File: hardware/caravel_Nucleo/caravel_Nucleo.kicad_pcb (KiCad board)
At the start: 2 copper layers, 67 x 92.4 mm, 80 parts, among them J1 USB_B_Micro - 10118193-0001LF, J10 Conn_01x09_Female, J2 Conn_01x02_Female, J3 Conn_01x02_Male, J4 Conn_01x04_Female, J5 Conn_01x02_Male, J6 Conn_01x02_Male, J7 Conn_01x06_Female, J8 Conn_01x03, J9 Conn_01x03, SW1 SW_Push - SKQGADE010, T1 Logo, T2 Logo, U1 FT232H, U10 MCP4661, U11 NUCLEO144-F429ZI, U2 SN74LVC1G125DCKR, U3 SN74LVC1G125DCKR, U4 MCP1319MT-29LE-OT, U5 TAR5SxxU_SOT353F, U6 TAR5SxxU_SOT353F, U7 W25Q32FVSS, U8 caravel_breakout, U9 MIC2211-AAYML-TR, X1 DSC6001_10MHZ, Y1 CSTNE12M0GH5L000R0

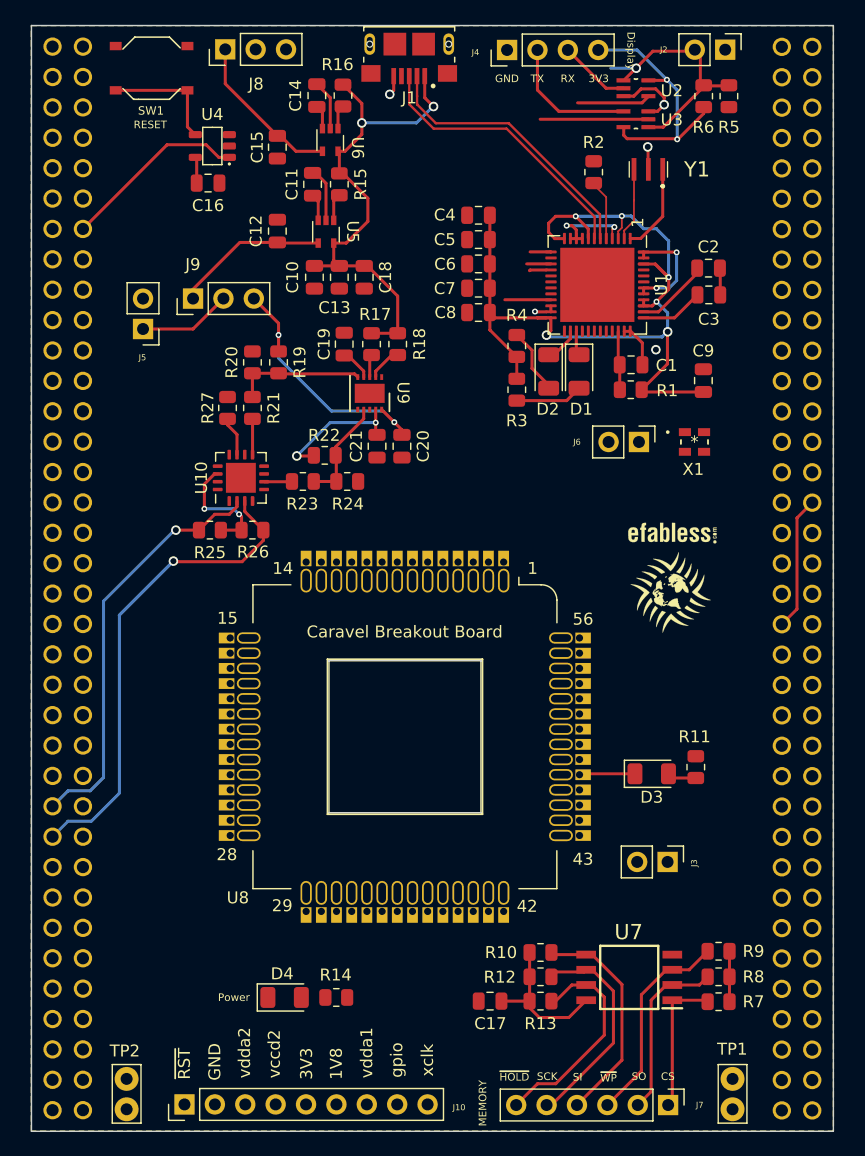
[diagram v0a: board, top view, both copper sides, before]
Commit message: [in review] update caravel board Nucleo-144 hat
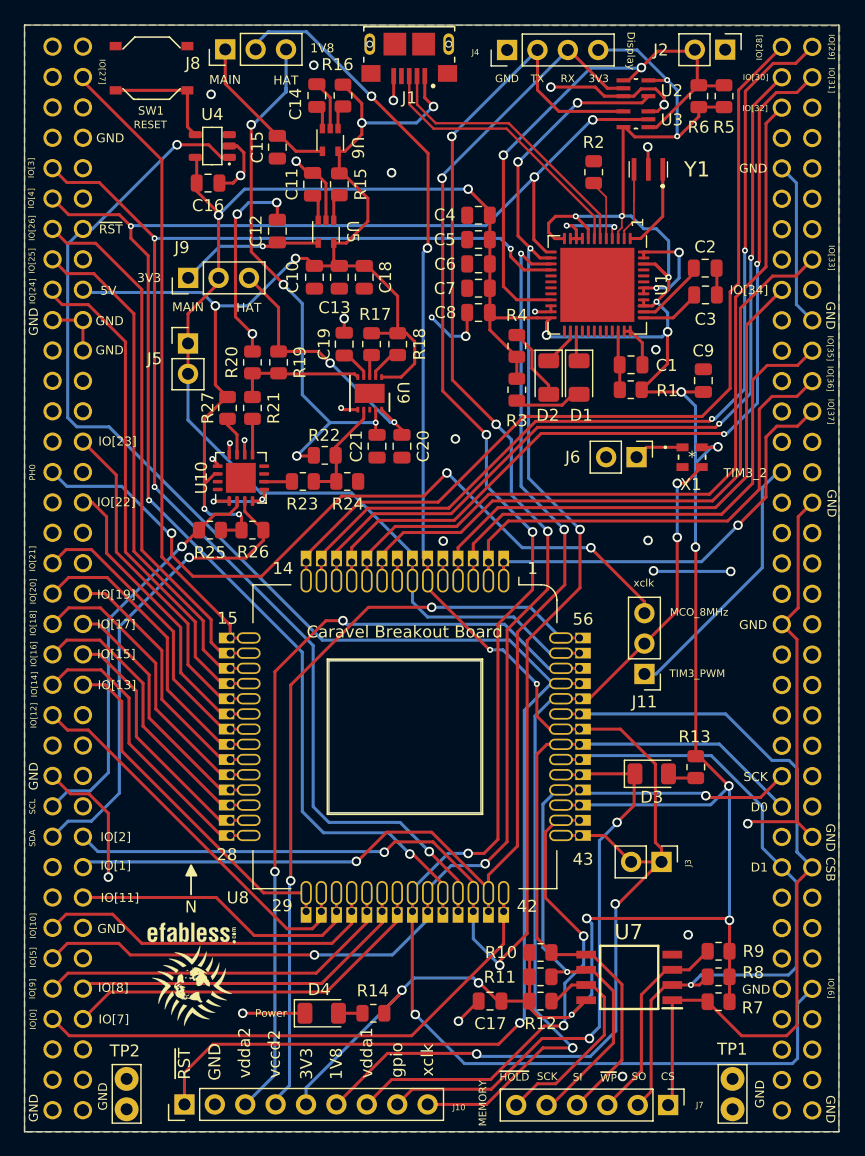
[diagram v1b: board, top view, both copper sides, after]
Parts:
- added J11: Conn_01x03, Connector_PinHeader_2.54mm:PinHeader_1x03_P2.54mm_Vertical, F.Cu at (146.9, 123.0)
- moved T2 52.3 mm to (109.0, 144.6)
- moved T1 51.8 mm to (109.0, 149.0)
- moved J5 3.95 mm to (108.7, 95.3), turned to 0 degrees
- moved D4 3.37 mm to (119.9, 151.3)
- moved R14 3.37 mm to (124.2, 151.3)
- moved J9 1.77 mm to (108.7, 89.9)
- moved X1 1.29 mm to (150.8, 104.9)
- moved J6 1.29 mm to (146.2, 104.9)
- moved J3 0.51 mm to (148.3, 138.7)
- moved D1 0.51 mm to (141.4, 98.2)
- moved D2 0.51 mm to (138.9, 98.2)
- moved R5 0.41 mm to (153.5, 74.7)
- moved R6 0.41 mm to (151.4, 74.7)
- moved C3 0.28 mm to (152.0, 91.3)
- moved C2 0.28 mm to (151.9, 89.1)
- renumbered R12 to R11, R13 to R12, R11 to R13
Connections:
- J10 pad 9: TIM3_CH2 -> xclk
- J3 pad 2: vccd1 -> vccd
- J4 pad 2: UART3_TX -> UART8_TX
- J4 pad 3: UART3_RX -> UART8_RX
- J5 pad 2: vddio -> vdda
- U1 pad 13: USB_SCK_TXD -> SPI5_SCK
- U1 pad 14: USB_SO_RXD -> SPI5_MISO
- U1 pad 15: USB_SI -> SPI5_MOSI
- U1 pad 16: USB_CS1 -> SPI5_CS
- U11 pad 1: UART3_TX -> unconnected-(U11-Pad1)
- U11 pad 136: unconnected-(U11-Pad136) -> UART8_RX
- U11 pad 2: UART3_RX -> unconnected-(U11-Pad2)
- U11 pad 29: unconnected-(U11-Pad29) -> PH0
- U11 pad 61: unconnected-(U11-Pad61) -> UART8_TX
- U2 pad 2: UART3_RX -> UART8_RX
- U2 pad 4: USB_SO_RXD -> SPI5_MISO
- U3 pad 2: USB_SCK_TXD -> SPI5_SCK
- U3 pad 4: UART3_TX -> UART8_TX
- U8 pad 36: UART3_RX -> UART8_RX
- U8 pad 37: UART3_TX -> UART8_TX
- U8 pad 38: USB_SCK_TXD -> SPI5_SCK
- U8 pad 39: USB_CS1 -> SPI5_CS
- U8 pad 40: USB_SO_RXD -> SPI5_MISO
- U8 pad 41: USB_SI -> SPI5_MOSI
- U8 pad 43: vccd1 -> vccd
- U8 pad 52: TIM3_CH2 -> xclk
- U8 pad 55: vddio -> vdda
- U8 pad 7: vddio -> vdda
- X1 pad 3: TIM3_CH2 -> xclk
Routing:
- net vdda: track 125.8 -> 328.0 mm, vias 8 -> 19
- net vccd: track 0.00 -> 142.7 mm, vias 0 -> 6
- net UART8_RX: track 0.00 -> 140.3 mm, vias 0 -> 5
- net SPI5_SCK: track 0.00 -> 132.6 mm, vias 0 -> 5
- net ~{RST}: track 15.6 -> 146.6 mm, vias 0 -> 2
- net SPI5_MISO: track 0.00 -> 130.2 mm, vias 0 -> 6
- net UART8_TX: track 0.00 -> 129.5 mm, vias 0 -> 5
- net GND: track 54.1 -> 174.2 mm, vias 9 -> 38
- net SPI5_CS: track 0.00 -> 114.8 mm, vias 0 -> 4
- net SPI5_MOSI: track 0.00 -> 99.4 mm, vias 0 -> 3
- net mprj_io[29]: track 0.00 -> 75.3 mm, vias 0 -> 2
- net mprj_io[28]: track 0.00 -> 73.7 mm
- net xclk: track 0.00 -> 71.9 mm, vias 0 -> 3
- net mprj_io[31]: track 0.00 -> 71.9 mm, vias 0 -> 2
- net mprj_io[30]: track 0.00 -> 70.1 mm, vias 0 -> 2
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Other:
- board size 67 x 92.4 mm -> 68.1 x 92.5 mm
- board text added: "5V"
- board text added: "CSB"
- board text added: "D0"
- board text added: "D1"
- board text added: "HAT"
- board text added: "IO[0]"
- board text added: "IO[10]"
- board text added: "IO[11]"
- board text added: "IO[12]"
- board text added: "IO[13]"
- board text added: "IO[14]"
- board text added: "IO[15]"
- board text added: "IO[16]"
- board text added: "IO[17]"
- board text added: "IO[18]"
- board text added: "IO[19]"
- board text added: "IO[1]"
- board text added: "IO[20]"
- board text added: "IO[21]"
- board text added: "IO[22]"
- board text added: "IO[23]"
- board text added: "IO[24]"
- board text added: "IO[25]"
- board text added: "IO[26]"
- board text added: "IO[27]"
- board text added: "IO[28]"
- board text added: "IO[29]"
- board text added: "IO[2]"
- board text added: "IO[30]"
- board text added: "IO[31]"
- board text added: "IO[32]"
- board text added: "IO[33]"
- board text added: "IO[34]"
- board text added: "IO[35]"
- board text added: "IO[36]"
- board text added: "IO[37]"
- board text added: "IO[3]"
- board text added: "IO[4]"
- board text added: "IO[5]"
- board text added: "IO[6]"
- board text added: "IO[7]"
- board text added: "IO[8]"
- board text added: "IO[9]"
- board text added: "MAIN"
- board text added: "MCO_8MHz"
- board text added: "N"
- board text added: "PH0"
- board text added: "SCL"
- board text added: "SDA"
- board text added: "TIM3_2"
- board text added: "TIM3_PWM"
